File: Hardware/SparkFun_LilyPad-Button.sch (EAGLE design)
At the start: 5 parts

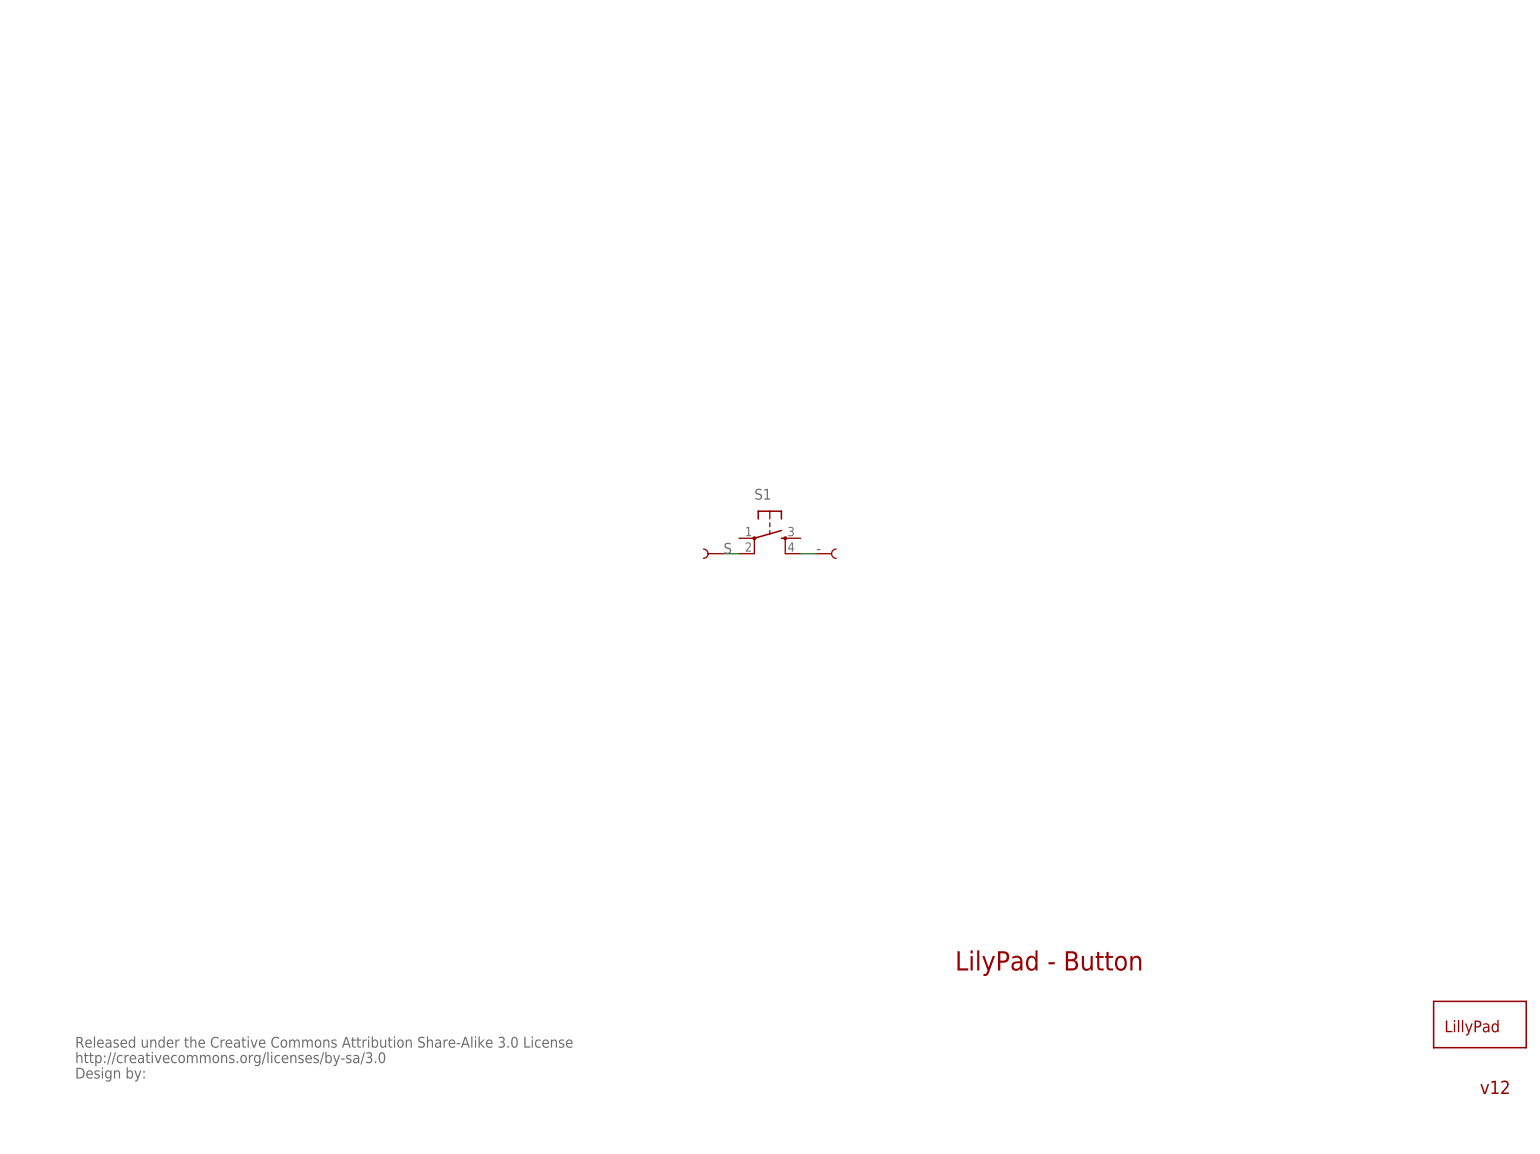
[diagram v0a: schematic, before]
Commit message: Initial Commit
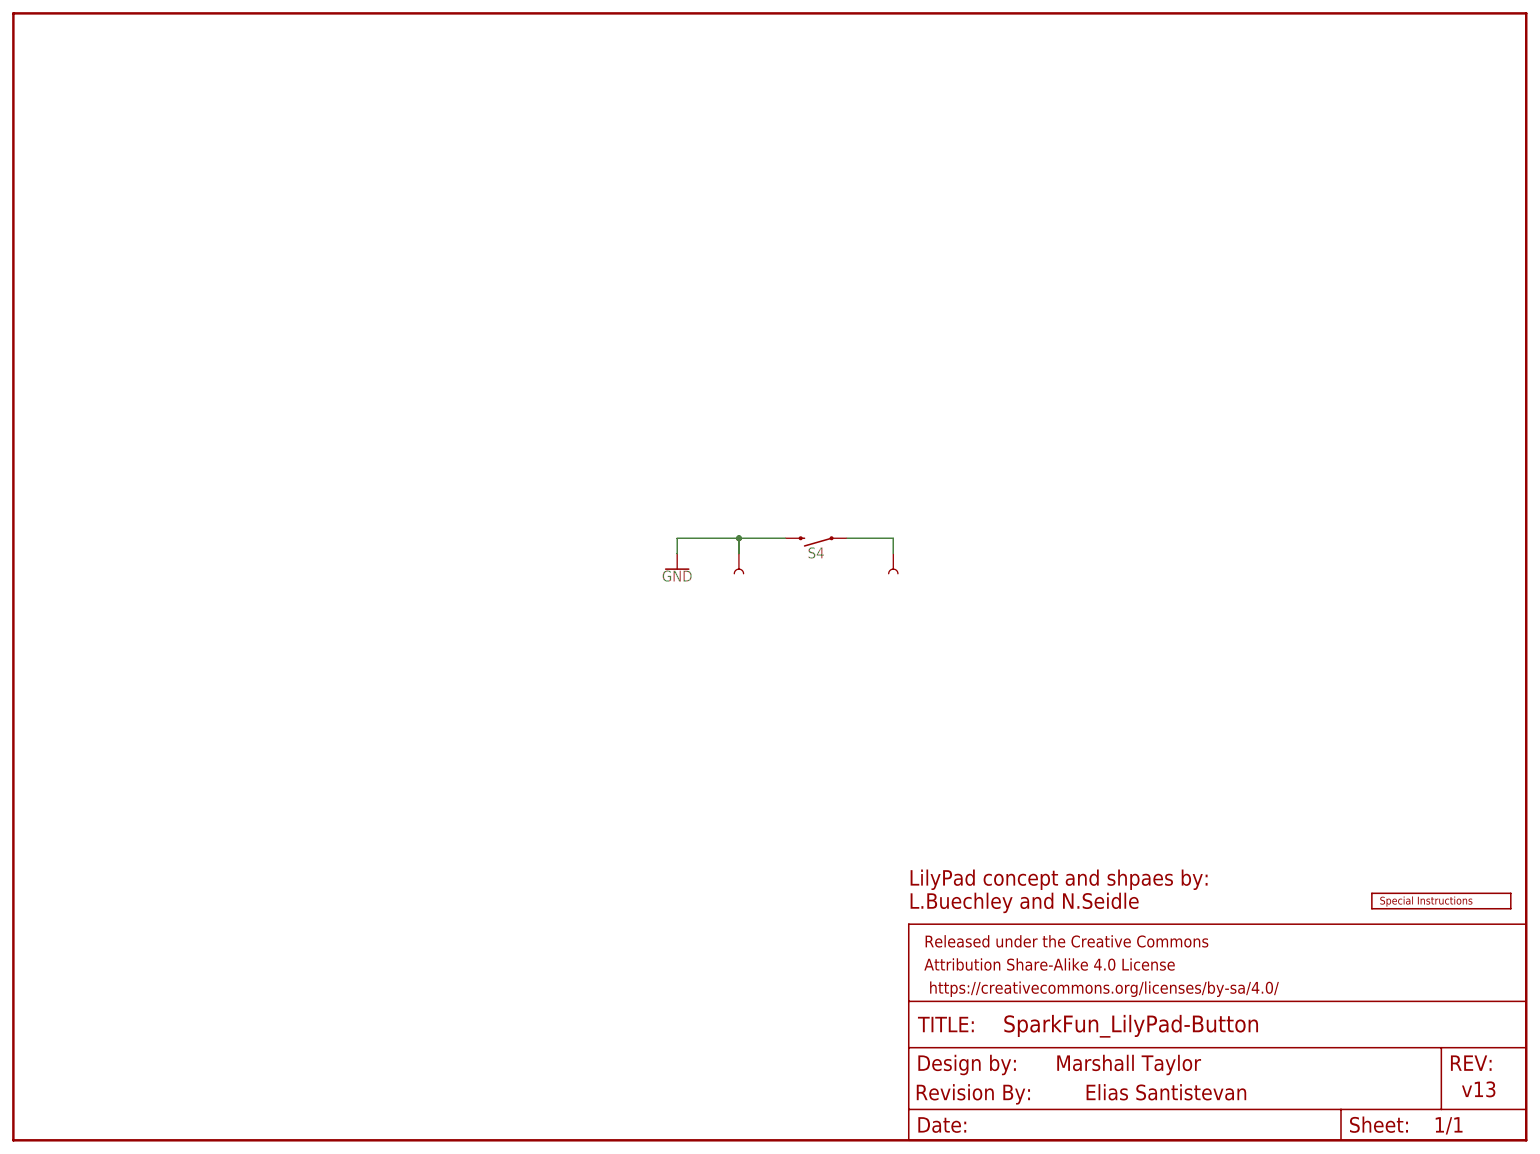
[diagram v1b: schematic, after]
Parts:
- removed BUTTON-, BUTTONS: SEWTAP8, LilyPad-Wearables:SEWTAP8
- removed LOGO1: LOGO-LPL, LilyPad-Wearables:LOGO-LPL
- removed S1: (no value), SparkFun:TAC_SWITCHSMD
- added FRAME2: FRAME-LETTER, SparkFun-Aesthetics:FRAME-LETTER
- added JP12, JP13: SEWTAP_MEDIUM-2SIDE, LilyPad-Wearables:SEWTAP_MEDIUM-2SIDE
- added S4: MOMENTARY-SWITCH-SPST-SMD-5.2-REDUNDANT, SparkFun-Switches:MOMENTARY-SWITCH-SPST-SMD-5.2-REDUNDANT
- U$1: value CREATIVE_COMMONS -> SPECIAL_INSTRUCTIONS-ORDERING; device SparkFun:CREATIVE_COMMONS -> SparkFun-Aesthetics:SPECIAL_INSTRUCTIONS-ORDERING
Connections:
- removed net -: BUTTON-.1, S1.4
- removed net S: BUTTONS.1, S1.2
- new net D4: JP12.1, S4.1
- new net GND: JP13.1, S4.2
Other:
- note added: "Elias Santistevan"
- note added: "LilyPad concept and shpaes by: L.Buechley and N.Seidle"
- note added: "Marshall Taylor"
- note added: "Revision By:"
- note added: "v13"
- note removed: "LilyPad - Button"
- note removed: "v12"
